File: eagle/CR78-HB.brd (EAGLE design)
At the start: 100 x 80 mm, 35 parts, among them Q1 2N3904, Q2 2N3904, Q3 2N3904

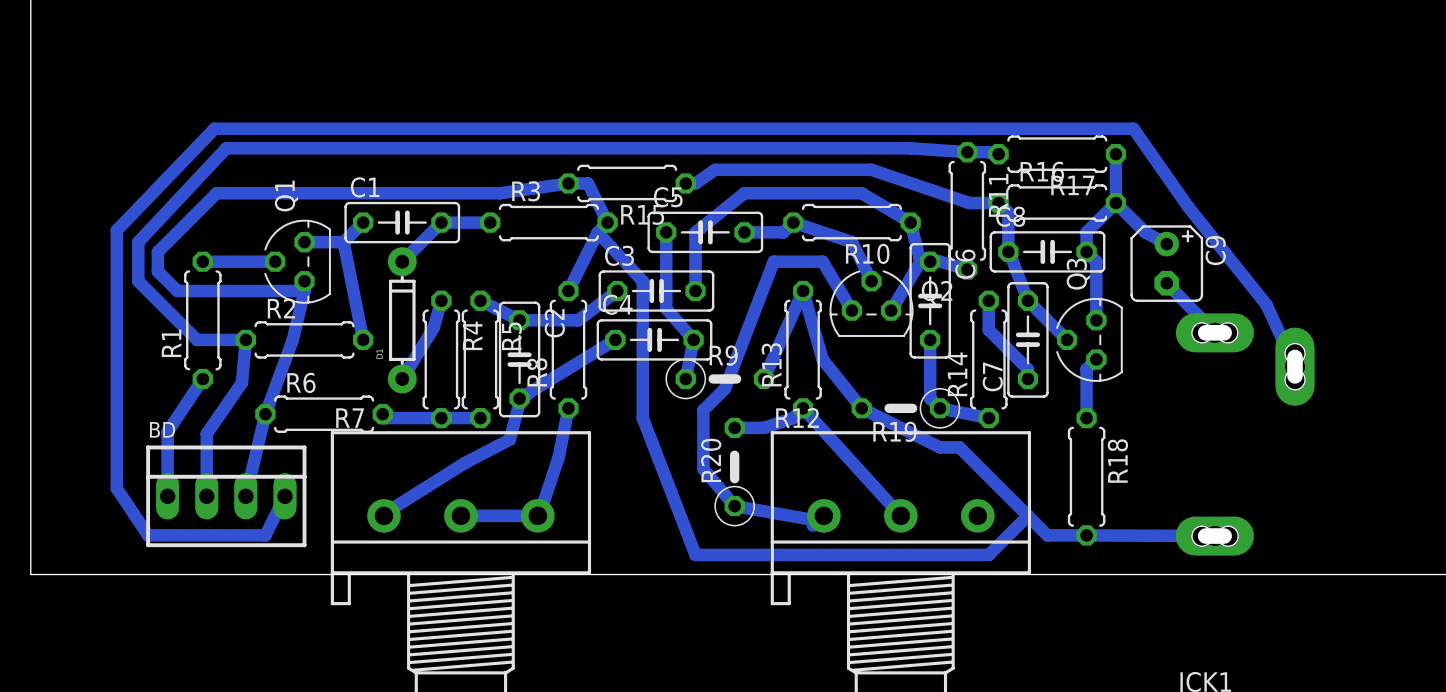
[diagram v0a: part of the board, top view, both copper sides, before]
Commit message: cutout
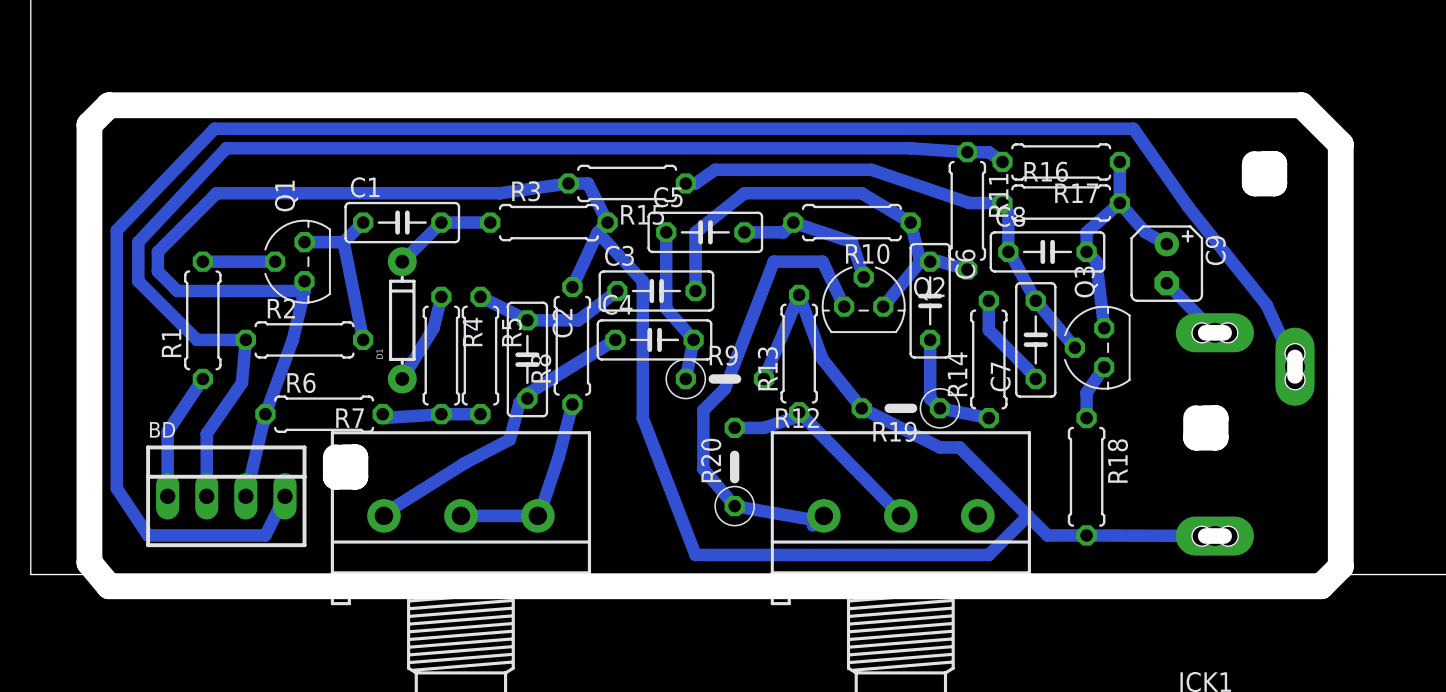
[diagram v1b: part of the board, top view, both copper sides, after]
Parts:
- moved Q3 0.72 mm to (69.7, 14.7)
- moved Q2 0.57 mm to (54.1, 17.4)
- moved R17 0.57 mm to (66.9, 26.8)
- moved C7 0.51 mm to (65.3, 15.2)
- moved C2 0.51 mm to (32.3, 14.0)
- moved R8 0.36 mm to (35.2, 14.9)
- moved R13 0.36 mm to (49.9, 14.4)
- moved R16 0.25 mm to (66.9, 24.1)
- moved R4 0.25 mm to (26.7, 14.2)
- moved R5 0.25 mm to (29.2, 14.2)
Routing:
- net GND: track 149.6 -> 148.8 mm
- net N$18: track 31.5 -> 32.2 mm
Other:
- board size 100 x 80 mm -> 100 x 80.8 mm
